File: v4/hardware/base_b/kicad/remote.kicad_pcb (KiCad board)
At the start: 2 copper layers, 111.8 x 100.3 mm, 31 parts, among them J12 Conn_01x04_Female, J16 Conn_01x04_Female, J19 Conn_01x03_Female, J2 Conn_01x12_Female, J20 Conn_01x04_Female, J3 Conn_01x16_Female, J5 Conn_01x03_Female, Q1 Q_NMOS_GDS, Q3 Q_NPN_EBC, SW1 SW_Push, SW2 SW_Push, SW4 SW_Push_Dual, U1 RFM95HW, U2 feather

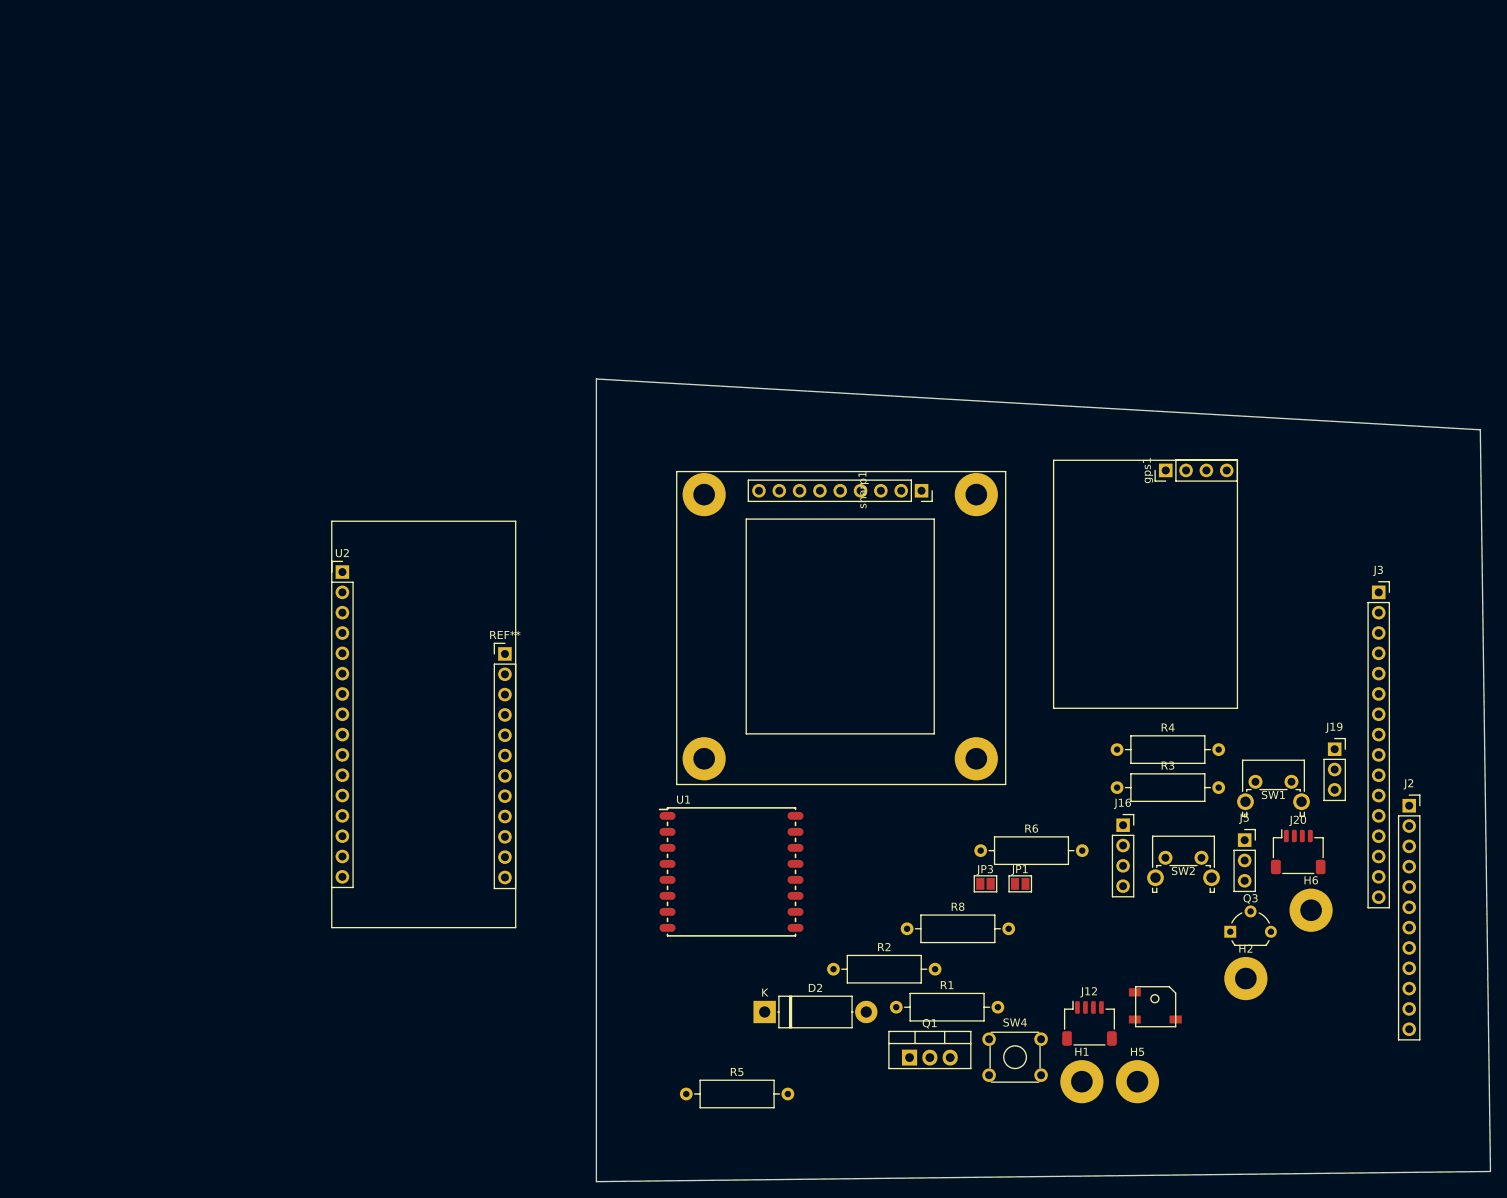
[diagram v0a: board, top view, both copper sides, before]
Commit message: update
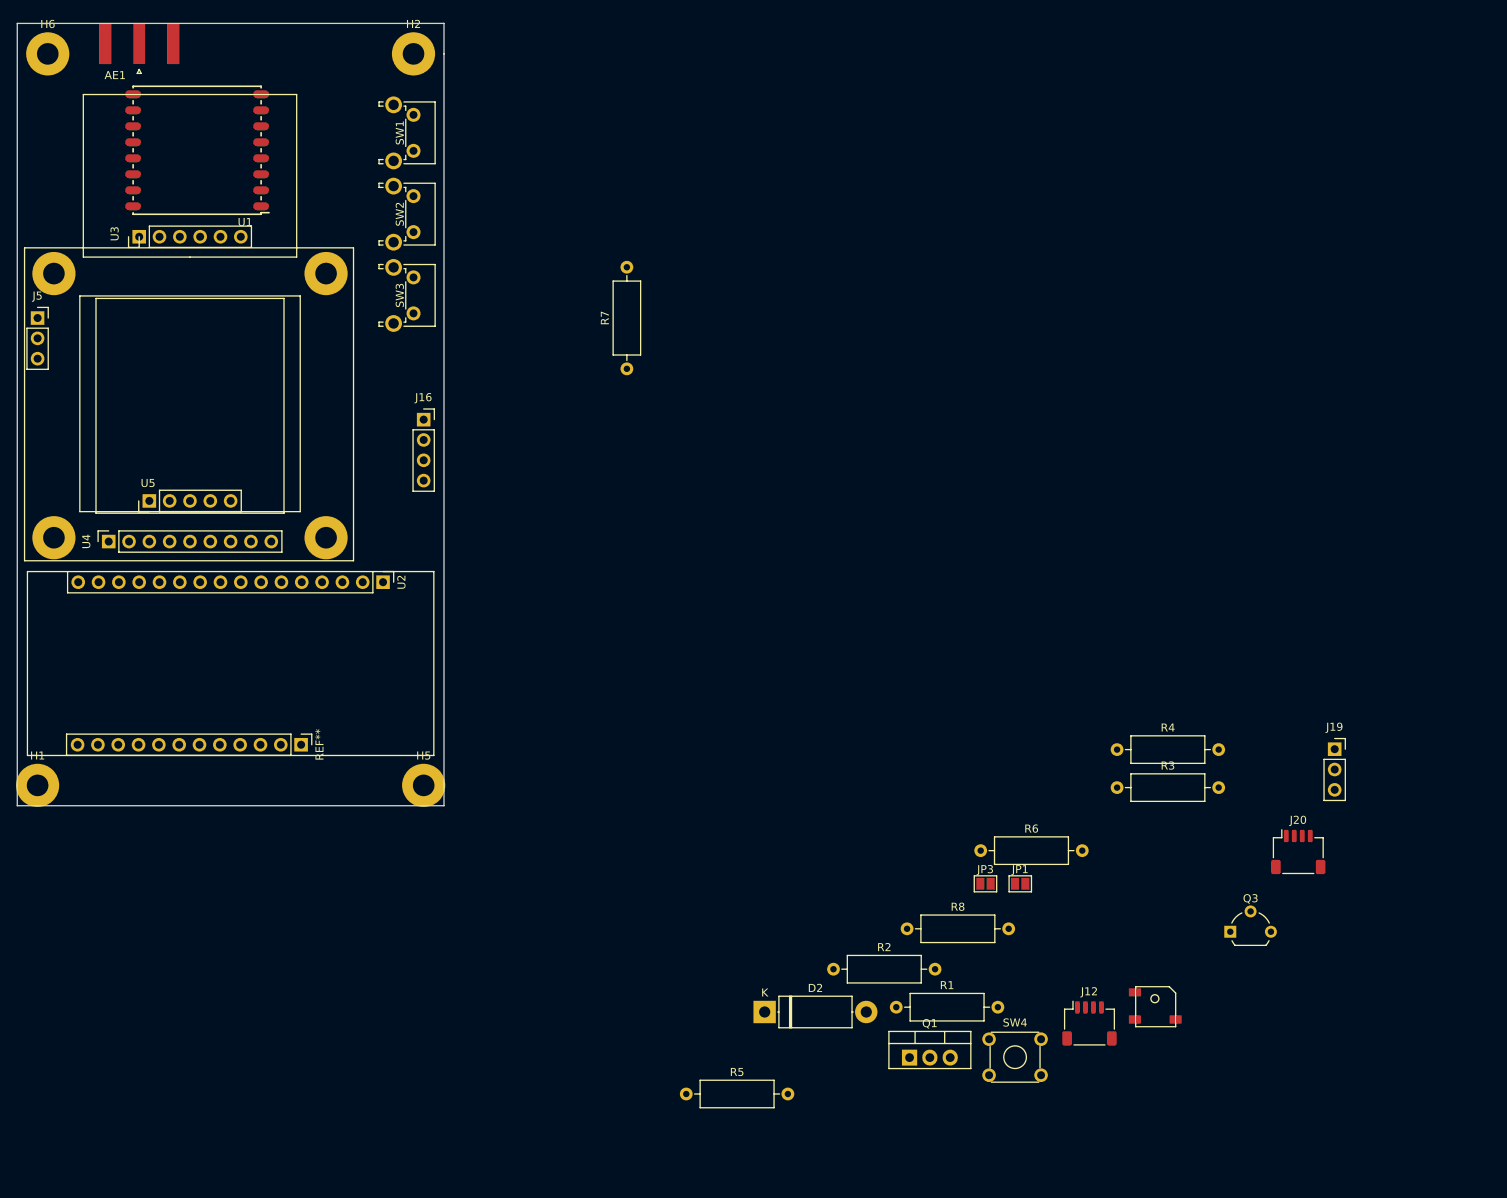
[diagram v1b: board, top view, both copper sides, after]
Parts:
- removed J2: Conn_01x12_Female, Connector_PinSocket_2.54mm:PinSocket_1x12_P2.54mm_Vertical
- removed J3: Conn_01x16_Female, Connector_PinSocket_2.54mm:PinSocket_1x16_P2.54mm_Vertical
- removed gps1: Conn_01x04_Female, footprints:gps_neo6_blue_0
- removed sharp1: Conn_01x09_Female, footprints:Display_adafruit_sharp_13
- added AE1: Antenna_Shield, Connector_Coaxial:SMA_Amphenol_132289_EdgeMount, F.Cu at (-16.5, -20.3)
- added R7: 4.7K, Resistor_THT:R_Axial_DIN0309_L9.0mm_D3.2mm_P12.70mm_Horizontal, F.Cu at (44.5, 20.3)
- added SW3: SW_Push, Button_Switch_THT:SW_Tactile_SPST_Angled_PTS645Vx58-2LFS, F.Cu at (17.8, 8.89)
- added U3: Adafruit_IMU_BNO005, footprints:IMU_Ada_BNO005, F.Cu at (-16.5, 3.81)
- added U4: Adafruit_Sharp_Display_1_3, footprints:Display_adafruit_sharp_13, F.Cu at (0.00, 41.9)
- added U5: neo-6m-black, footprints:gps_neo6m_black, F.Cu at (-15.2, 36.8)
- moved H6 190.8 mm to (-27.9, -19.1)
- moved J5 164.4 mm to (-29.2, 14.0)
- moved H2 155.5 mm to (17.8, -19.1)
- moved H1 135.7 mm to (-29.2, 72.4)
- moved SW1 134.3 mm to (17.8, -11.4), turned to 270 degrees
- moved SW2 125.2 mm to (17.8, -1.27), turned to 270 degrees
- moved J16 101.1 mm to (19.1, 26.7)
- moved H5 96.6 mm to (19.1, 72.4)
- moved U1 91.6 mm to (-1.27, 0.00), turned to 180 degrees
- moved U2 5.24 mm to (14.0, 47.0), turned to 270 degrees
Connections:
- J5 pad 2: EN -> (no net)
- U2 pad 11: (no net) -> SCL
- U2 pad 12: (no net) -> SDA
- U2 pad 17: (no net) -> A0
- U2 pad 20: (no net) -> A3
- U2 pad 21: (no net) -> A4
- U2 pad 22: (no net) -> A5
- U2 pad 26: (no net) -> RX_D0
- U2 pad 27: (no net) -> TX_D1
- U2 pad 28: (no net) -> DW
- U2 pad 8: (no net) -> D9
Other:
- board size 111.8 x 100.3 mm -> 53.3 x 97.8 mm
